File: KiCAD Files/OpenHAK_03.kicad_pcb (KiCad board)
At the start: 4 copper layers, 38.1 x 25.4 mm, 52 parts, among them P1 Harwin M52 Series, P2 USB_OTG, U1 rfd_77101, U2 MAX30100, U3 MIC5365-1.8YMT-TZ, U4 BMI160, U5 MCP73831T-2ATI/OT, U6 MIC5365-3.0YMT-TZ, U7 TXS0102DQER

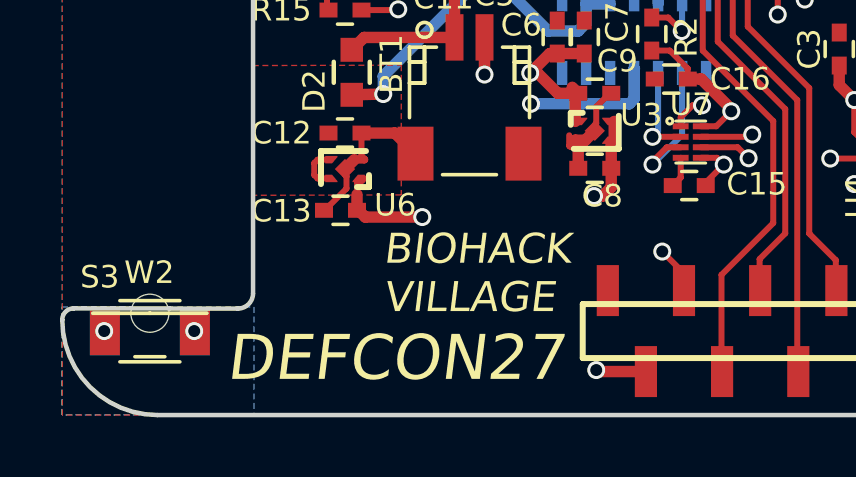
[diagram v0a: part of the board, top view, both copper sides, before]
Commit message: Added PDFs of the top and bottom
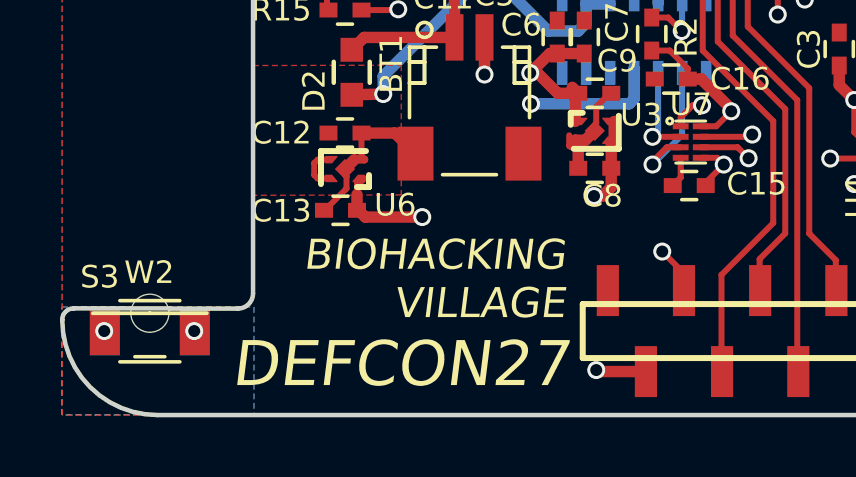
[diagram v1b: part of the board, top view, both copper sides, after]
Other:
- board text added: "BIOHACKING VILLAGE"
- board text removed: "BIOHACK VILLAGE"
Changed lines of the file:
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@@
       (xy -3.228344 8.4504)) (layer B.SilkS) (width 0.01))
   )
-  (gr_text "BIOHACK\nVILLAGE" (at 132.04 106.16) (layer F.SilkS)
-    (effects (font (size 1 1) (thickness 0.2) italic) (justify left))
+  (gr_text "BIOHACKING\nVILLAGE" (at 138.12 106.36) (layer F.SilkS)
+    (effects (font (size 1 1) (thickness 0.2) italic) (justify right))
   )
   (gr_text DEFCON27 (at 131.3 99.62 90) (layer B.SilkS)
@@
     (effects (font (size 1 1) (thickness 0.25)) (justify mirror))
   )
-  (gr_text DEFCON27 (at 132.44088 108.99386) (layer F.SilkS)
+  (gr_text DEFCON27 (at 132.61 109.2) (layer F.SilkS)
     (effects (font (size 1.5 1.5) (thickness 0.3) italic))
   )
